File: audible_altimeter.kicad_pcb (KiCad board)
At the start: 2 copper layers, 52 x 29 mm, 61 parts, among them CON1 BUQ2-USB-MICRO-B, IC1 BUQ2-ATXMEGA128A4U-A, P1 CONN_2, P2 SERIAL, P3 POWER, Q1 NPN-SOT23, U1 MCP7940M, U10 CNT, U11 DWN, U12 2SMPB-01-01, U13 FLASH_MEMORY, U14 MCP4017, U15 SPDT-SWITCH, U16 MPU-9250, U2 MCP73831-SOT-23-5, U3 NCP4681-SC-70, U4 UP, U5 MPL3115A2, U6 MS5805-02BA01, U7 LS013B4DN04, U8 CSS-0575A-SMT, U9 TAG-CONNECT-ATMEL-PDI-CONNECT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, X1 CRYSTAL

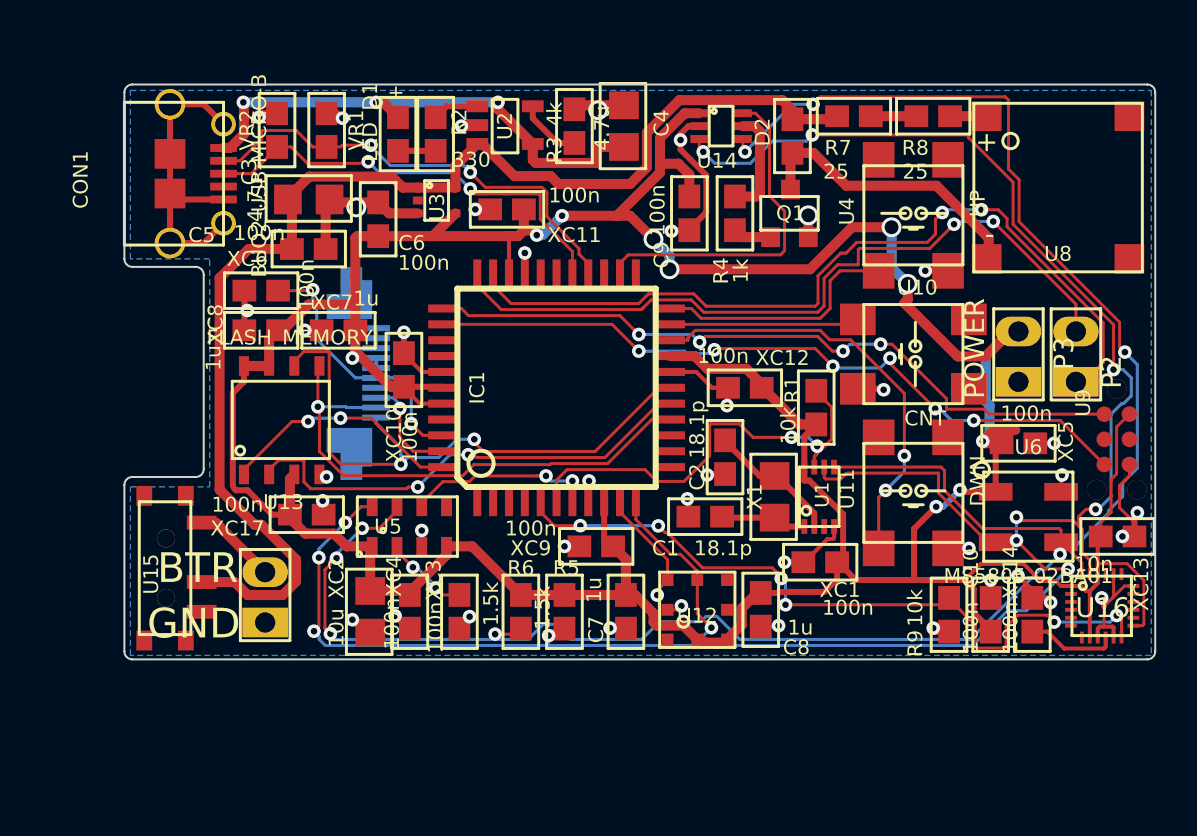
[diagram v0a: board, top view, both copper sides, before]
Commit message: Some changes?
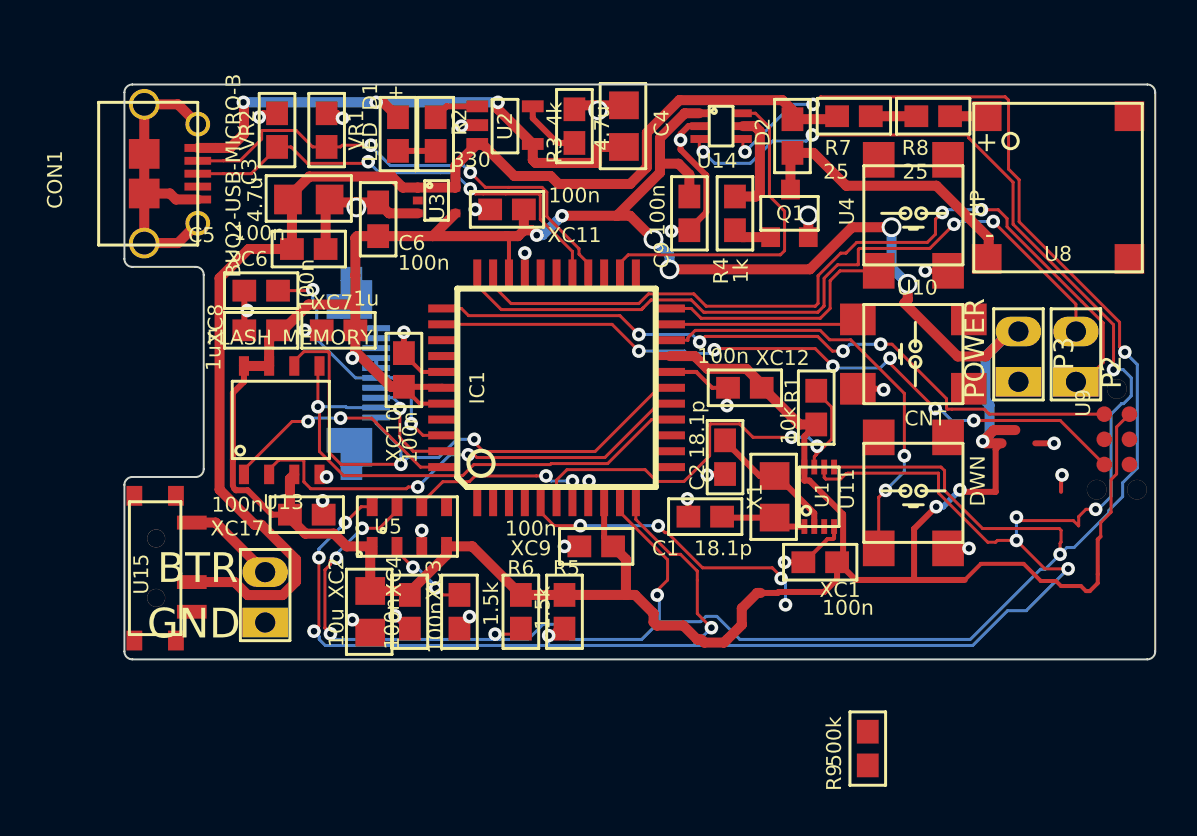
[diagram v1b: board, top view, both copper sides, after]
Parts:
- removed C10, XC14, XC5: 100n, buq2:SM0603
- removed C7, C8: 1u, buq2:SM0603
- removed U12: 2SMPB-01-01, buq2:2SMPB-01-01
- removed U16: MPU-9250, buq2:24QFN-3MM-3MM
- removed U6: MS5805-02BA01, buq2:MS5805-02BA01
- removed XC13: 10n, buq2:SM0603
- R9: value 10k -> 500k
- moved R9 7.90 mm to (173.2, 129.7)
- moved CON1 1.30 mm to (139.4, 100.7)
- moved U15 0.50 mm to (137.3, 120.6)
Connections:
- net /Accelerometer/I2C_SCL renamed /Barometer/I2C_SCL
- net /Accelerometer/I2C_SDA renamed /Barometer/I2C_SDA
- IC1 pad 41: (no net) -> /Battery/BATTERY_SENSE
- IC1 pad 5: /MCU/ACC_INT -> (no net)
- R9 pad 1: GND -> /Battery/BATTERY
- R9 pad 2: /MCU/ACC_INT -> /Battery/BATTERY_SENSE
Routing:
- net /MCU/ACC_INT: track 36.9 -> 0.00 mm, vias 6 -> 0
- net GND: track 89.1 -> 67.7 mm, vias 40 -> 28
- net (no net): track 0.00 -> 17.4 mm, vias 0 -> 6
- net /Battery/+3.3V: track 209.1 -> 198.1 mm
- net Net-(U16-Pad10): track 4.55 -> 0.00 mm
- net /Barometer/I2C_SCL: track 122.5 -> 119.9 mm
- net /Barometer/I2C_SDA: track 117.8 -> 115.5 mm
- net /MCU/D-: track 23.6 -> 24.9 mm
- net /MCU/D+: track 22.3 -> 23.6 mm
- net /Battery/+5V: track 26.5 -> 27.8 mm
- removed copper zone on B.Cu, net GND
